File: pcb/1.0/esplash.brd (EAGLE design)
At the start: 101 x 67.6 mm, 57 parts, among them Q5 BCX70SMD, Q6 BCX70SMD, U1 ESP-WROOM-32, Y1 ECS-.327-12.5-13X

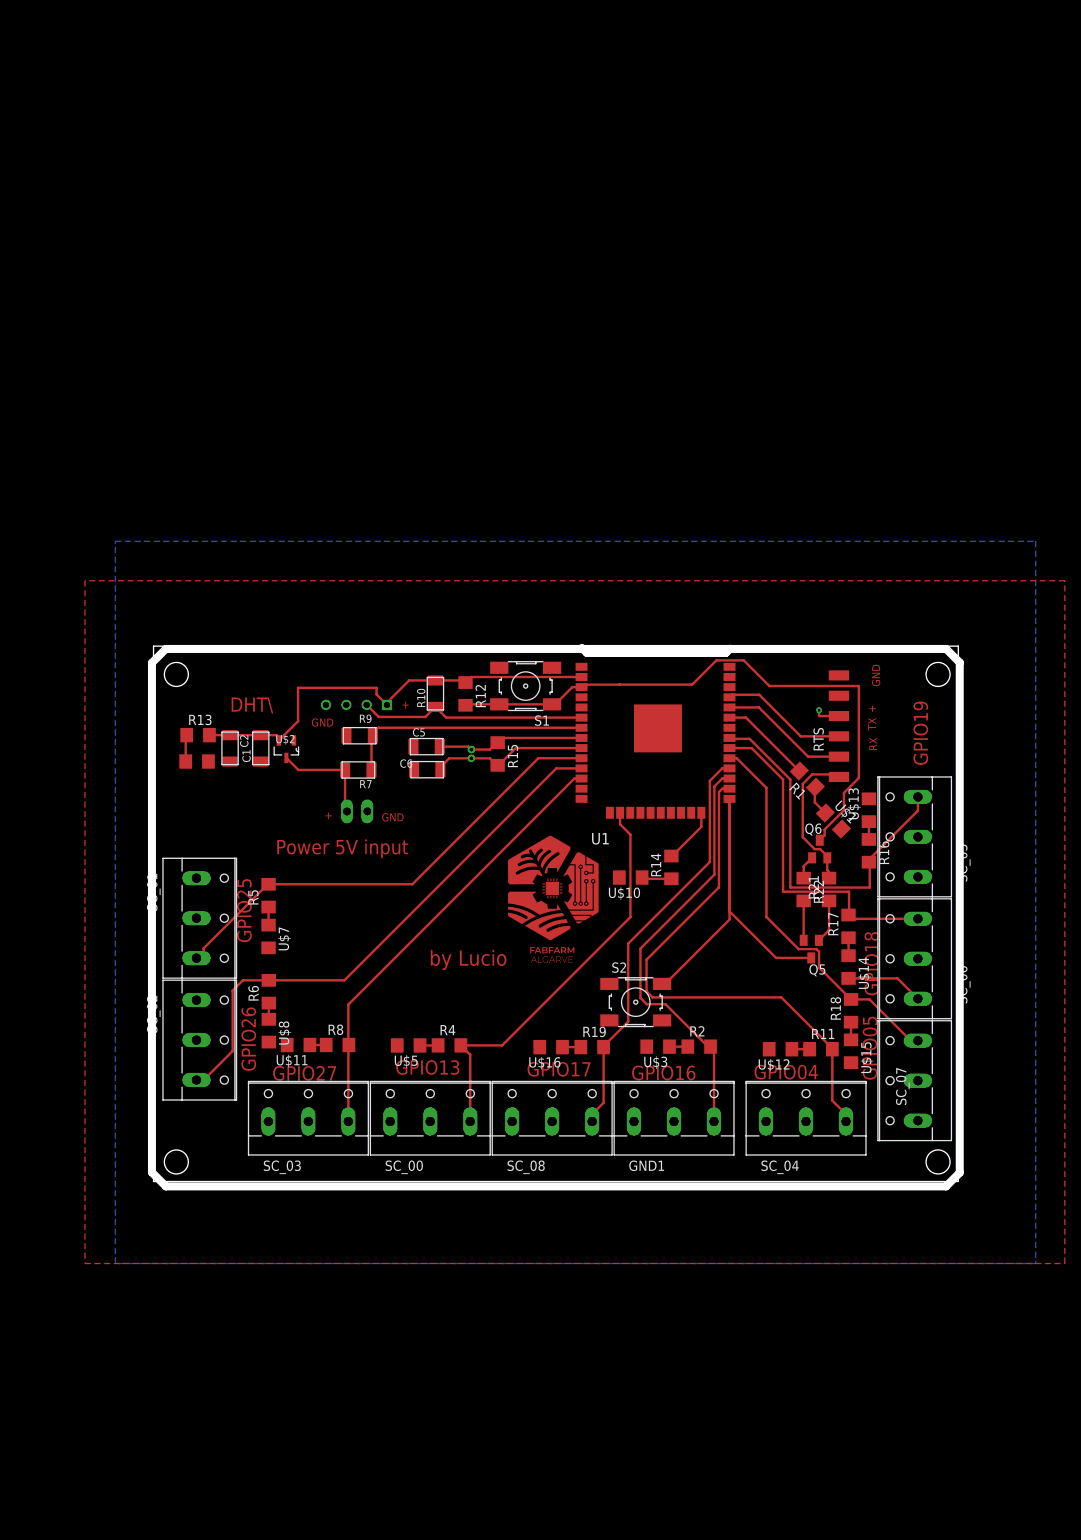
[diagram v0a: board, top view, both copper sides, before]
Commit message: pcb updates
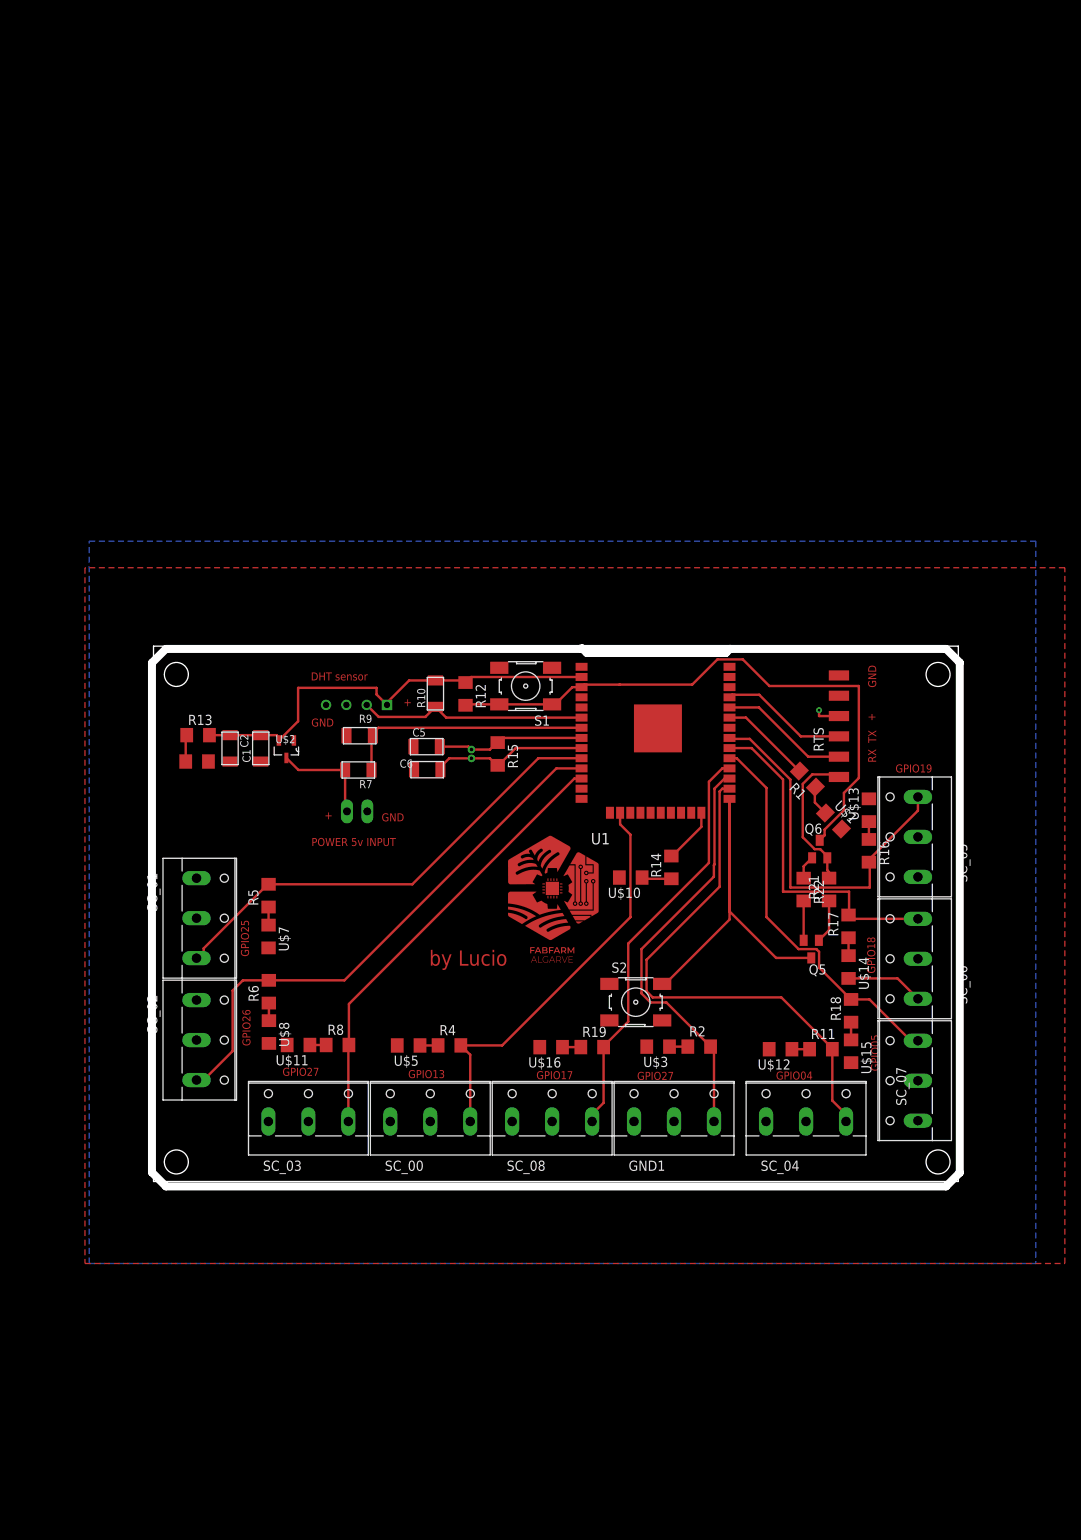
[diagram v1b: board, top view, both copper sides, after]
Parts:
- moved U$8 0.17 mm to (14.1, 22.6)
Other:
- board text added: "DHT sensor"
- board text added: "POWER 5v INPUT"
- board text removed: "DHT\"
- board text removed: "GPIO16"
- board text removed: "Power 5V input"

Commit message: new board
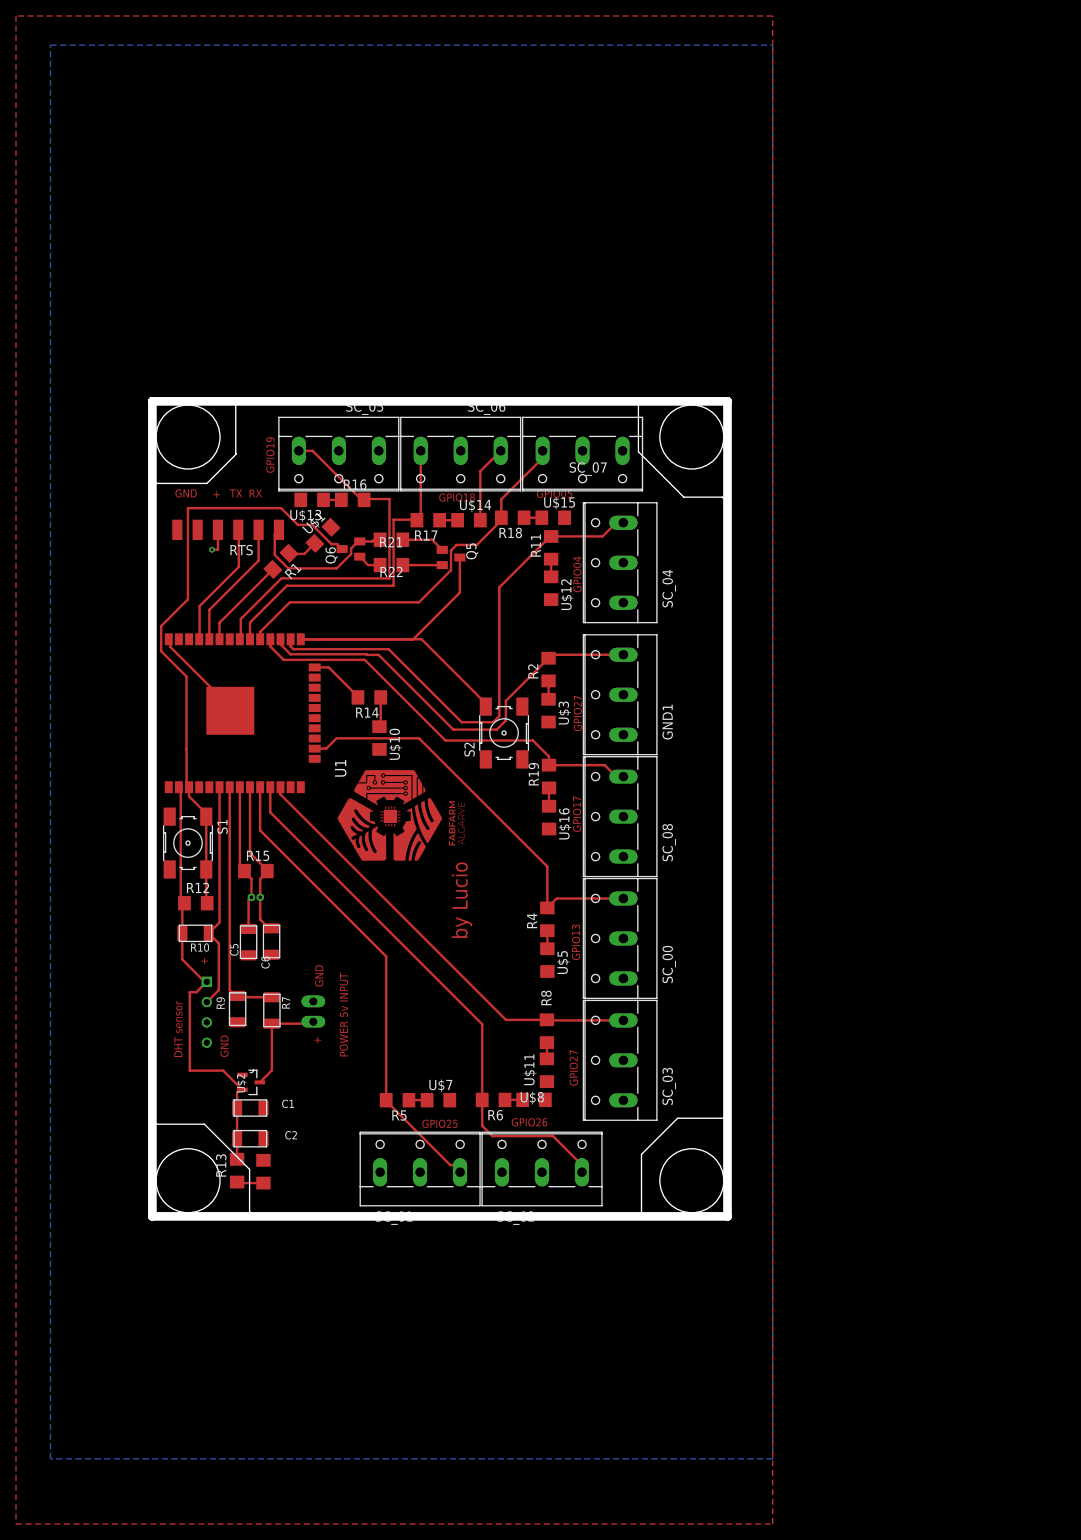
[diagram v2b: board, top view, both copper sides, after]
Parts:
- moved SC_07 87.5 mm to (53.3, 94.0), turned to 180 degrees
- moved SC_05 85.2 mm to (22.9, 94.0), turned to 180 degrees
- moved SC_06 83.6 mm to (38.1, 94.0), turned to 180 degrees
- moved RTS 80.2 mm to (9.01, 85.4), turned to 90 degrees
- moved U$13 79.7 mm to (19.5, 89.1), turned to 180 degrees
- moved R16 78.1 mm to (24.6, 89.1), turned to 0 degrees
- moved U$15 76.4 mm to (49.7, 86.9), turned to 0 degrees
- moved R18 74.8 mm to (44.6, 86.9), turned to 180 degrees
- moved U$14 73.3 mm to (39.1, 86.6), turned to 0 degrees
- moved U$1 73.2 mm to (20.9, 84.7), turned to 45 degrees
- moved R17 73.1 mm to (34.0, 86.6), turned to 180 degrees
- moved SC_04 72.7 mm to (57.1, 81.3), turned to 90 degrees
- moved R1 71.2 mm to (15.6, 81.4), turned to 225 degrees
- moved R11 71.2 mm to (49.4, 83.1), turned to 90 degrees
- moved R21 70.1 mm to (29.4, 84.2), turned to 180 degrees
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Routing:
- net GND: track 9.73 -> 21.3 mm
- net GPIO1/TXD0: track 16.4 -> 15.8 mm
- net GPIO17/VALVE_RELAY08: track 51.8 -> 52.4 mm
- net GPIO16/CURRENT_SENSE: track 52.7 -> 53.2 mm
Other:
- board size 101 x 67.6 mm -> 72 x 102 mm
